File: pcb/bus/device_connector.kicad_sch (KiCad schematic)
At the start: 3 parts, among them J201 Conn_02x10_Row_Letter_First

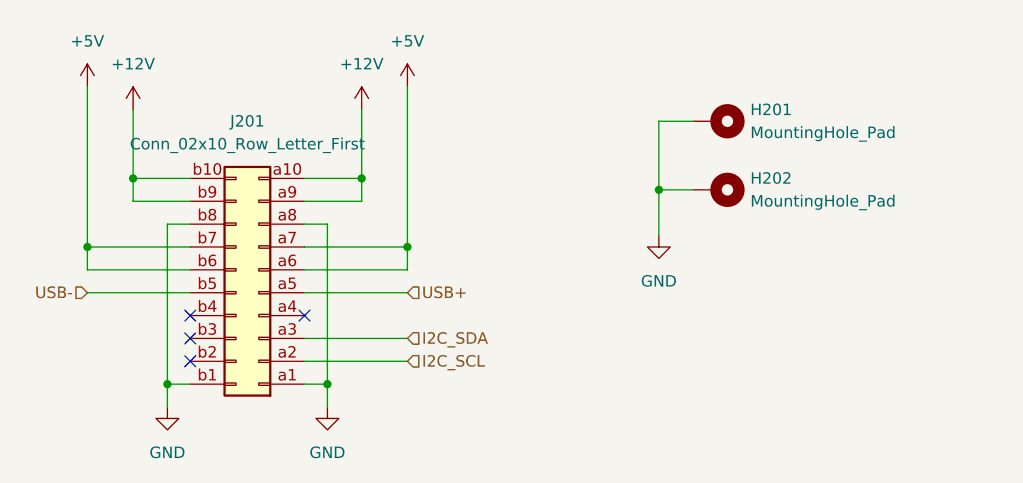
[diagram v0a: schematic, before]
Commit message: update bus pcb
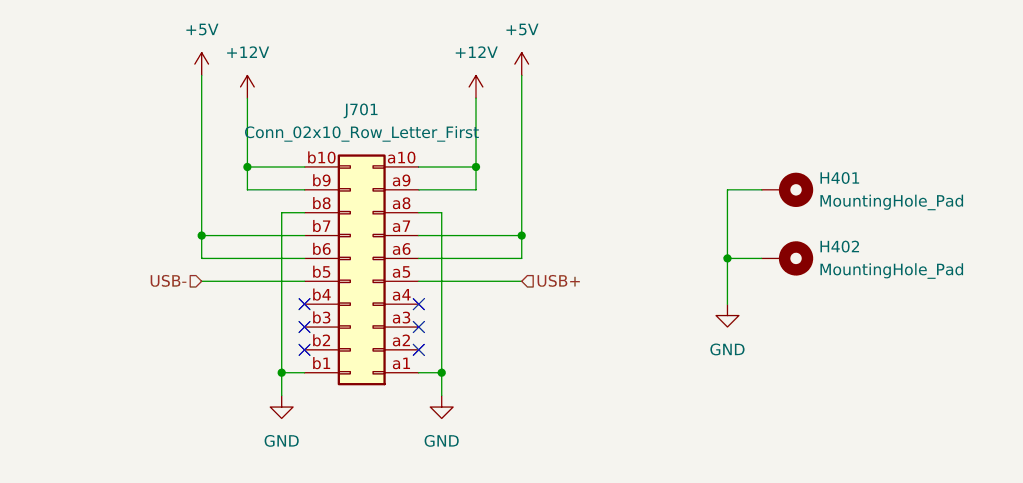
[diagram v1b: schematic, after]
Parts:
- removed H201, H202: MountingHole_Pad, MountingHole:MountingHole_3.2mm_M3_Pad_Via, symbol Mechanical:MountingHole_Pad
- removed J201: Conn_02x10_Row_Letter_First, PRJ:PCN10-20P-2.54DSA, symbol Connector_Generic:Conn_02x10_Row_Letter_First
- added H401, H402: MountingHole_Pad, MountingHole:MountingHole_3.2mm_M3_Pad_Via, symbol Mechanical:MountingHole_Pad
- added J701: Conn_02x10_Row_Letter_First, PRJ:PCN10-20P-2.54DSA, symbol Connector_Generic:Conn_02x10_Row_Letter_First
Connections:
- net +12V: now also J701.a10 (Pin_a10), J701.a9 (Pin_a9), J701.b10 (Pin_b10), J701.b9 (Pin_b9)
- net +5V: now also J701.a6 (Pin_a6), J701.a7 (Pin_a7), J701.b6 (Pin_b6), J701.b7 (Pin_b7)
- net GND: now also H401.1, H402.1, J701.a1 (Pin_a1), J701.a8 (Pin_a8), J701.b1 (Pin_b1), J701.b8 (Pin_b8)
- net USB+: now also J701.a5 (Pin_a5)
- net USB-: now also J701.b5 (Pin_b5)
- no-connect marks 4 -> 6
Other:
- title: Bus Connector -> (none)
